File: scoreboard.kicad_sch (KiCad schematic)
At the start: 14 parts, among them J601 8P8C_LED_Shielded, U601 PCA9615DP

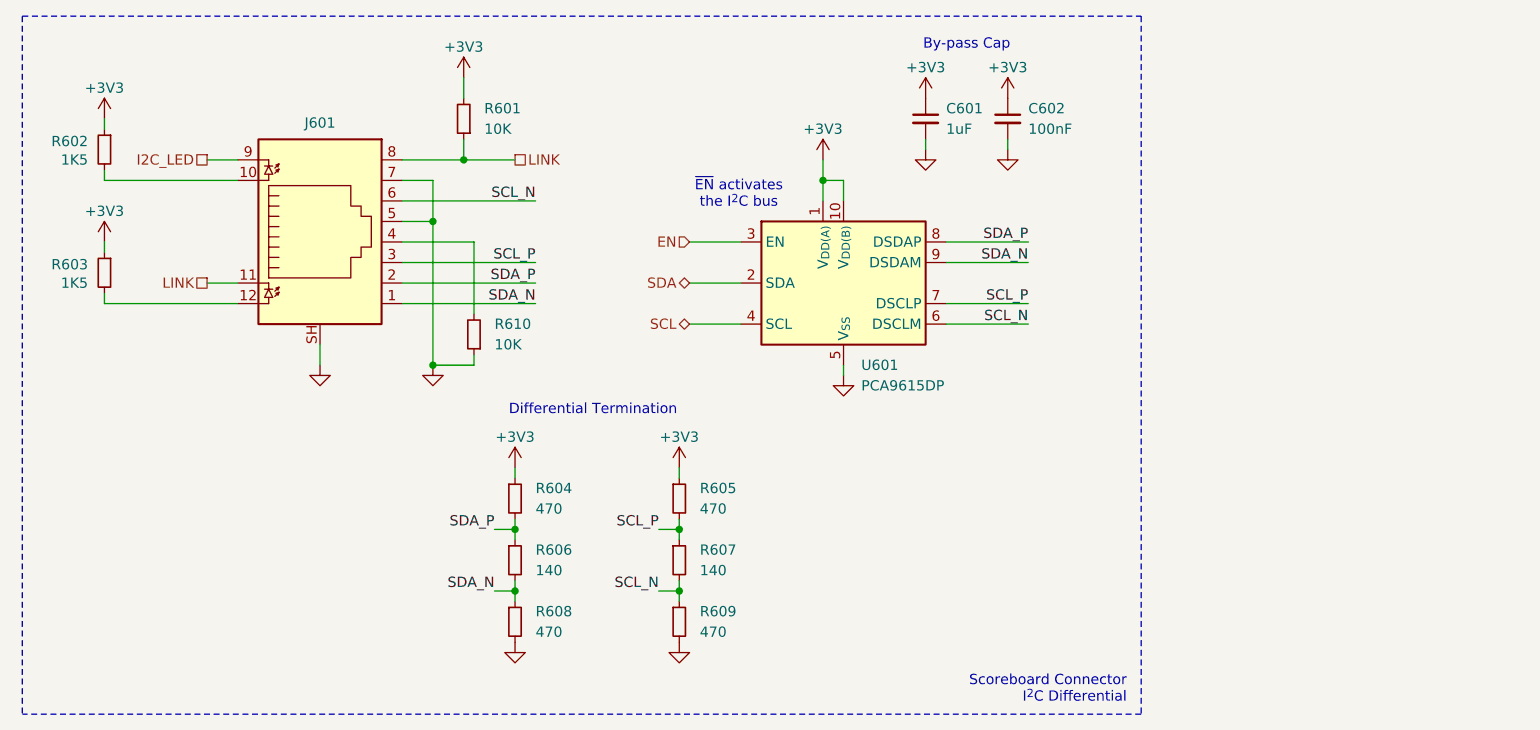
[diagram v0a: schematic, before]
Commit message: update pdf
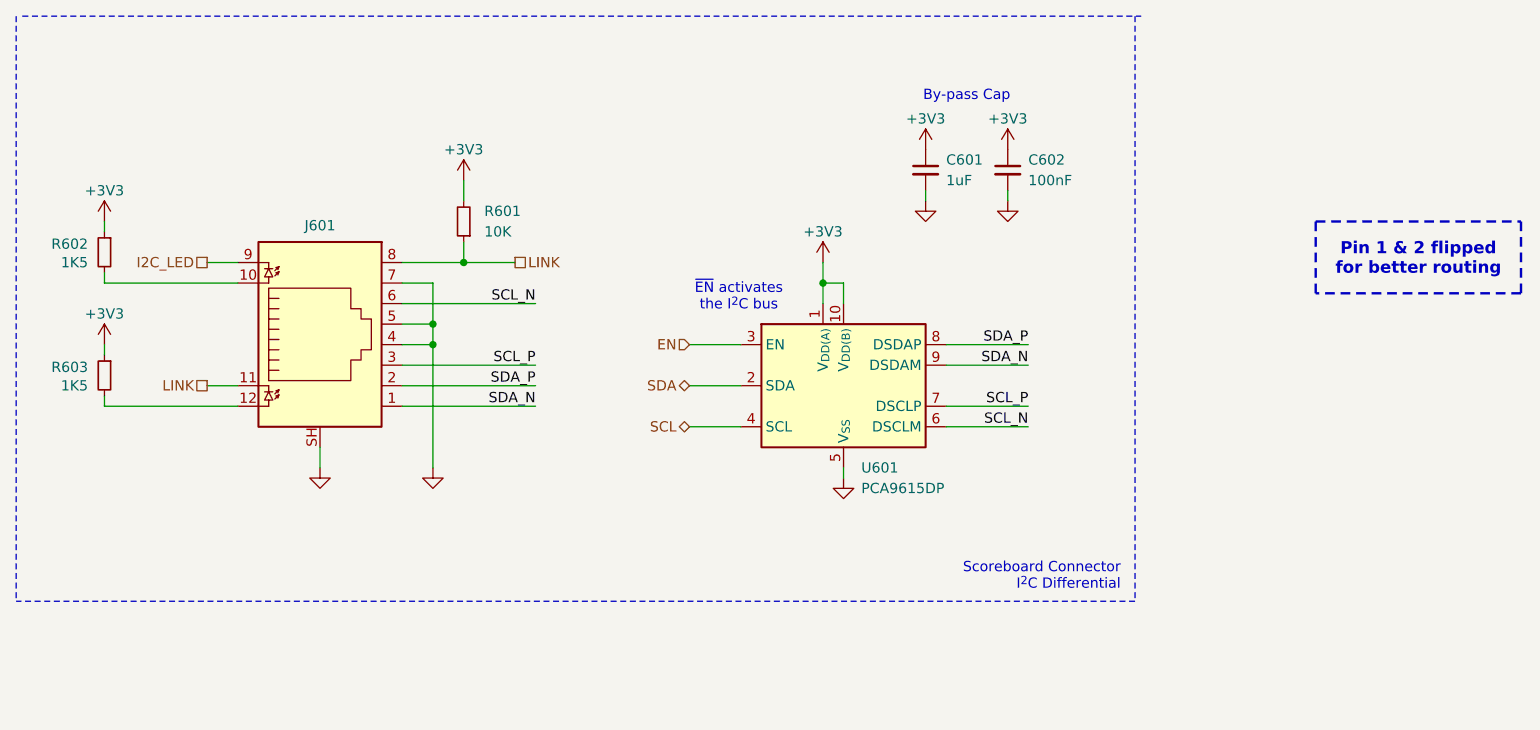
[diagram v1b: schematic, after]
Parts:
- removed R604, R605, R608, R609: 470, Resistor_SMD:R_0603_1608Metric, symbol Device:R_Small
- removed R606, R607: 140, Resistor_SMD:R_0603_1608Metric, symbol Device:R_Small
- removed R610: 10K, Resistor_SMD:R_0603_1608Metric, symbol Device:R_Small
- U601: now left out of the parts list
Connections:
- net GND: now also J601.4
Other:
- note removed: "Differential Termination"
- moved on the sheet: C601, C602, J601, R601, R602, R603, U601
